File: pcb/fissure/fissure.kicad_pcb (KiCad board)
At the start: 2 copper layers, 109 x 96 mm, 82 parts, among them J1 AudioJack4, J10 Conn_01x03, J11 Conn_01x03, J2 AudioJack4, J3 Conn_01x04, J4 Conn_01x04, J5 Conn_01x03, J6 Conn_01x03, J7 Conn_01x04, J8 Conn_01x04, J9 Conn_01x04, K1 KEYSW, K10 KEYSW, K11 KEYSW, K12 KEYSW, K13 KEYSW, K14 KEYSW, K15 KEYSW, K16 KEYSW, K17 KEYSW, K18 KEYSW, K19 KEYSW, K2 KEYSW, K20 KEYSW, K3 KEYSW, K4 KEYSW, K5 KEYSW, K6 KEYSW, K7 KEYSW, K8 KEYSW, K9 KEYSW, SW1 SW_PUSH, SW2 SW_SPDT, SW3 SW_SPDT, SW4 SW_PUSH, U1 nice_nano, U2 MT25QL128ABA1ESE, U3 MT25QL128ABA1ESE

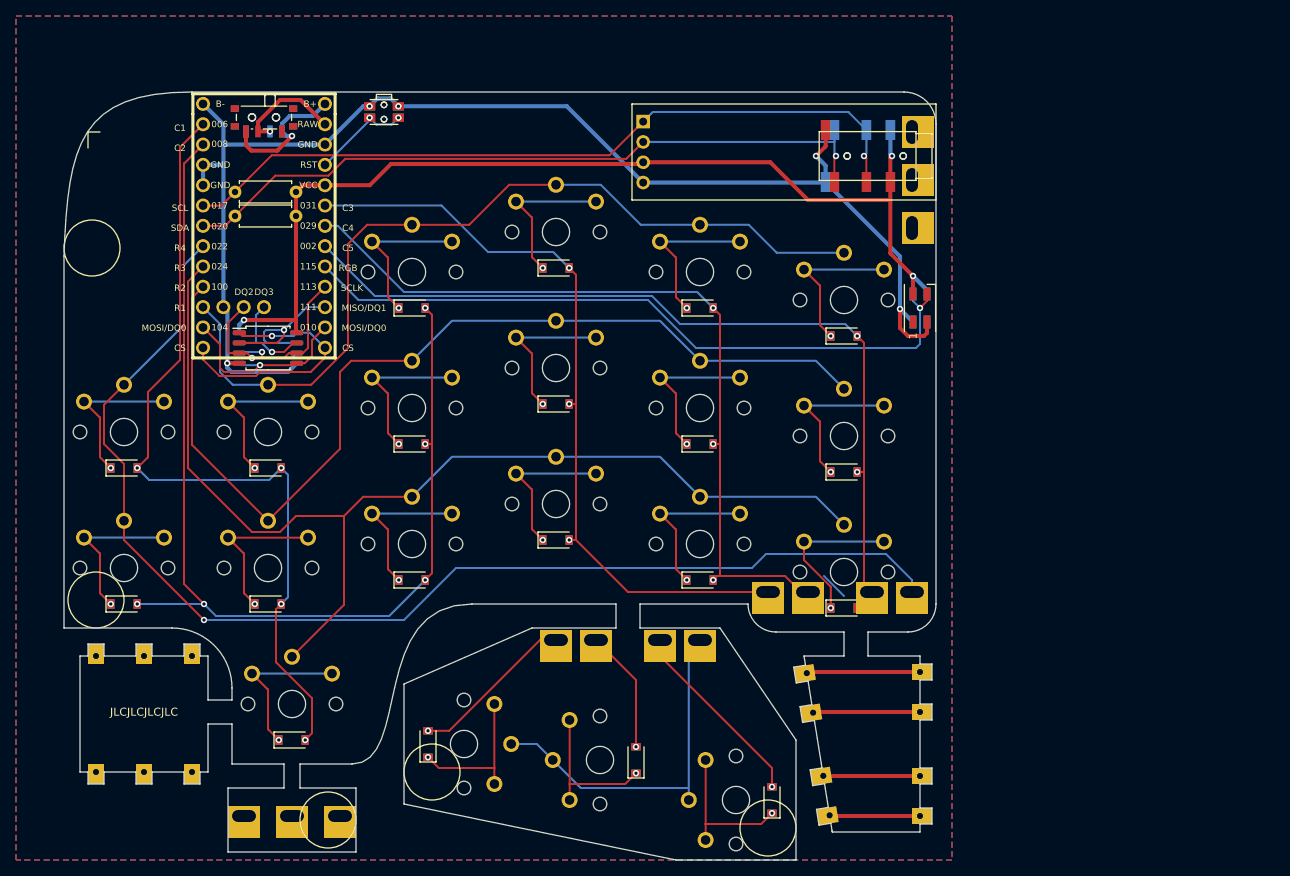
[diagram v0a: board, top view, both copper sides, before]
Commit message: v3.1
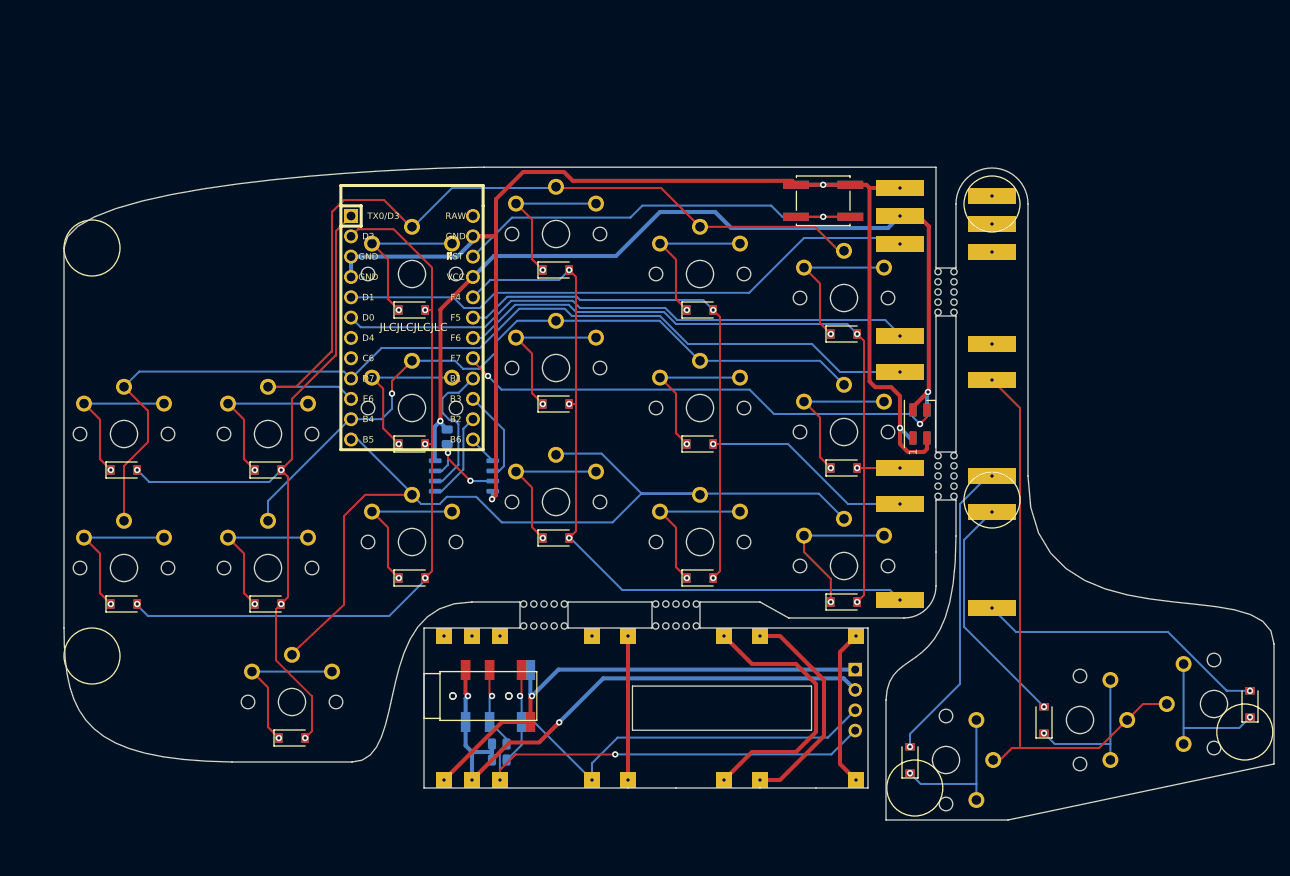
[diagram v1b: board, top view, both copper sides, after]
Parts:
- removed J10: Conn_01x03, fissure:feet
- removed J11: Conn_01x03, fissure:feet-conn
- removed J7, J8: Conn_01x04, fissure:bridge
- removed the SW2 at (51.0, 48.5)
- removed SW3: SW_SPDT, Button_Switch_SMD:SW_SPDT_PCM12
- removed U3: MT25QL128ABA1ESE, Package_SO:SOP-8_5.28x5.23mm_P1.27mm
- added R3: R, Resistor_SMD:R_0805_2012Metric, B.Cu at (73.9, 88.1)
- added REF**: breakaway-mousebites, Keebio-Parts:breakaway-mousebites, F.Cu at (135.0, 93.0)
- added REF**: breakaway-mousebites, Keebio-Parts:breakaway-mousebites, F.Cu at (137.5, 93.0)
- added REF**: breakaway-mousebites, Keebio-Parts:breakaway-mousebites, F.Cu at (135.0, 70.0)
- added REF**: breakaway-mousebites, Keebio-Parts:breakaway-mousebites, F.Cu at (137.5, 70.0)
- added REF**: breakaway-mousebites, Keebio-Parts:breakaway-mousebites, F.Cu at (102.5, 108.8)
- added REF**: breakaway-mousebites, Keebio-Parts:breakaway-mousebites, F.Cu at (86.0, 108.8)
- added REF**: breakaway-mousebites, Keebio-Parts:breakaway-mousebites, F.Cu at (102.5, 112.0)
- added REF**: breakaway-mousebites, Keebio-Parts:breakaway-mousebites, F.Cu at (86.0, 112.0)
- D35, D37, D39, K18, K19, K20, U2: moved to B.Cu
- D36, D38, D40: moved to F.Cu
- J3: value Conn_01x04 -> Conn_01x08; moved to F.Cu
- J4: value Conn_01x04 -> Conn_01x08; footprint fissure:bridge-conn -> fissure:bridge; moved to F.Cu
- J5: value Conn_01x03 -> Conn_01x08; footprint fissure:feet -> fissure:bridge-conn; moved to B.Cu
- J6: value Conn_01x03 -> Conn_01x08; footprint fissure:feet-conn -> fissure:bridge
- R1, R2: footprint Resistor_THT:R_Axial_DIN0207_L6.3mm_D2.5mm_P7.62mm_Horizontal -> Resistor_SMD:R_0805_2012Metric; moved to B.Cu
- SW1: footprint Button_Switch_SMD:SW_SPST_EVQP7C -> Button_Switch_SMD:SW_SPST_EVQQ2
- SW2: renamed from SW4; footprint Button_Switch_SMD:SW_SPST_EVQP7C -> Button_Switch_SMD:SW_SPST_EVQQ2
- U1: value nice_nano -> ProMicro; footprint nice-nano-kicad:nice_nano -> Keebio-Parts:ArduinoProMicro
- moved J5 110.2 mm to (142.0, 85.5), turned to 90 degrees
- moved D35 102.9 mm to (174.2, 121.5)
- moved D36 102.9 mm to (174.2, 121.5)
- moved K18 93.9 mm to (169.8, 121.5)
- moved J1 90.0 mm to (73.0, 120.5), turned to 90 degrees
- moved J2 90.0 mm to (73.0, 120.5), turned to 270 degrees
- moved J9 85.7 mm to (126.5, 127.0), turned to 180 degrees
- moved R1 73.5 mm to (80.4, 126.5), turned to 0 degrees
- moved R2 72.6 mm to (80.4, 128.5), turned to 0 degrees
- moved J6 64.9 mm to (101.0, 113.0), turned to 180 degrees
- moved K19 60.2 mm to (153.0, 123.5)
- moved SW1 56.0 mm to (120.9, 58.6)
- moved SW2 56.0 mm to (120.9, 58.6)
- moved D37 51.2 mm to (148.5, 123.5)
- moved D38 51.2 mm to (148.5, 123.5)
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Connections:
- D35 pad 2: Net-(D35-Pad2) -> thumb_COL3
- D36 pad 2: Net-(D35-Pad2) -> thumb_COL3
- D37 pad 2: Net-(D37-Pad2) -> thumb_COL4
- D38 pad 2: Net-(D37-Pad2) -> thumb_COL4
- D39 pad 2: Net-(D39-Pad2) -> thumb_COL5
- D40 pad 2: Net-(D39-Pad2) -> thumb_COL5
- J1 pad R1: SDA -> bridge_SDA
- J1 pad R2: VCC -> bridge_VCC
- J1 pad S: GND -> bridge_GND
- J1 pad T: SCL -> bridge_SCL
- J2 pad R1: SDA -> bridge_SDA
- J2 pad R2: VCC -> bridge_VCC
- J2 pad S: GND -> bridge_GND
- J2 pad T: SCL -> bridge_SCL
- J4 pad 1: Net-(D35-Pad2) -> Net-(J4-Pad1)
- J4 pad 2: Net-(D37-Pad2) -> Net-(J4-Pad2)
- J4 pad 3: Net-(D39-Pad2) -> Net-(J4-Pad3)
- J5 pad 1: Net-(J5-Pad1) -> thumb_COL3
- J5 pad 2: Net-(J5-Pad2) -> thumb_COL4
- J5 pad 3: Net-(J5-Pad3) -> thumb_COL5
- J6 pad 1: Net-(J6-Pad1) -> Net-(J4-Pad1)
- J6 pad 2: Net-(J6-Pad2) -> Net-(J4-Pad2)
- J6 pad 3: Net-(J6-Pad3) -> Net-(J4-Pad3)
- J9 pad 1: SDA -> bridge_GND
- J9 pad 2: SCL -> bridge_VCC
- J9 pad 3: VCC -> bridge_SCL
- J9 pad 4: GND -> bridge_SDA
- K18 pad 1: Net-(J4-Pad4) -> thumb_ROW4
- K19 pad 1: Net-(J4-Pad4) -> thumb_ROW4
- K20 pad 1: Net-(J4-Pad4) -> thumb_ROW4
- R1 pad 1: VCC -> bridge_VCC
- R1 pad 2: SDA -> bridge_SDA
- R2 pad 1: VCC -> bridge_VCC
- R2 pad 2: SCL -> bridge_SCL
- U1 pad 11: MOSI_DQ0 -> ROW2
- U1 pad 12: CS -> ROW3
- U1 pad 24: MCU_RAW -> RAW
- U1 pad 7: ROW4 -> Net-(U1-Pad7)
- U1 pad 8: ROW3 -> Net-(U1-Pad8)
- U1 pad 9: ROW2 -> ROW4
- U2 pad 3: DQ2 -> Net-(R3-Pad2)
- U2 pad 7: DQ3 -> Net-(R3-Pad2)
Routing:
- net thumb_ROW4: track 0.00 -> 73.1 mm
- net bridge_VCC: track 0.00 -> 72.9 mm, vias 0 -> 2
- net bridge_SDA: track 0.00 -> 62.9 mm, vias 0 -> 2
- net bridge_GND: track 0.00 -> 62.2 mm, vias 0 -> 1
- net bridge_SCL: track 0.00 -> 61.7 mm, vias 0 -> 1
- net RST: track 12.5 -> 57.2 mm, vias 2 -> 1
- net COL2: track 133.5 -> 91.9 mm, vias 5 -> 4
- net thumb_COL5: track 0.00 -> 38.4 mm, vias 0 -> 1
- net thumb_COL3: track 0.00 -> 36.5 mm, vias 0 -> 1
- net ROW2: track 125.3 -> 90.8 mm, vias 0 -> 1
- net Net-(J4-Pad3): track 0.00 -> 34.0 mm
- net thumb_COL4: track 0.00 -> 29.9 mm, vias 0 -> 1
- net CS: track 31.6 -> 3.68 mm, vias 1 -> 0
- net Net-(J4-Pad2): track 0.00 -> 27.6 mm
- net ROW4: track 151.8 -> 124.8 mm, vias 1 -> 0
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- removed copper zone on B.Cu, net GND
- removed copper zone on F.Cu, net GND
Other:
- board size 109 x 96 mm -> 151.2 x 81.6 mm
- rule pad_to_mask_clearance: 0.051 -> 0
- board text added: "4.7k"
- board text removed: "C1"
- board text removed: "C2"
- board text removed: "C3"
- board text removed: "C4"
- board text removed: "C5"
- board text removed: "CS"
- board text removed: "DQ2"
- board text removed: "DQ3"
- board text removed: "MISO/DQ1"
- board text removed: "MOSI/DQ0"
- board text removed: "R1"
- board text removed: "R2"
- board text removed: "R3"
- board text removed: "R4"
- board text removed: "RGB"
- board text removed: "SCL"
- board text removed: "SCLK"
- board text removed: "SDA"
